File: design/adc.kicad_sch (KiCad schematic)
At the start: 27 parts, among them J6 JUMPER_DFS/GAIN, U12 TLV431ACDBZR, U13 AD9214

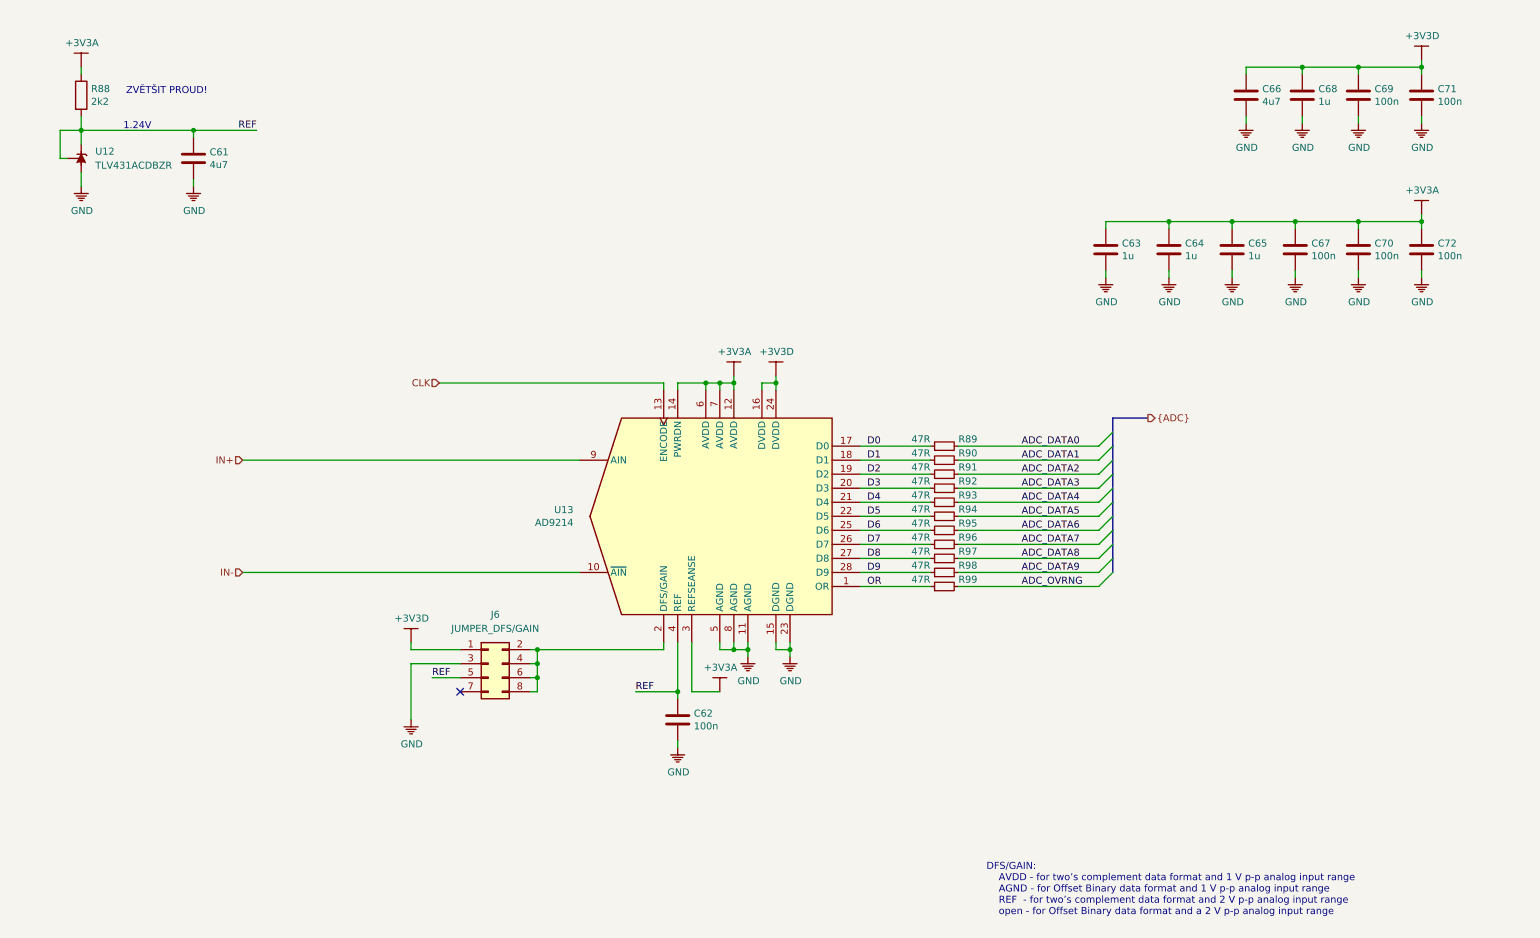
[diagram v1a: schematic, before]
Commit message: Updated schematic
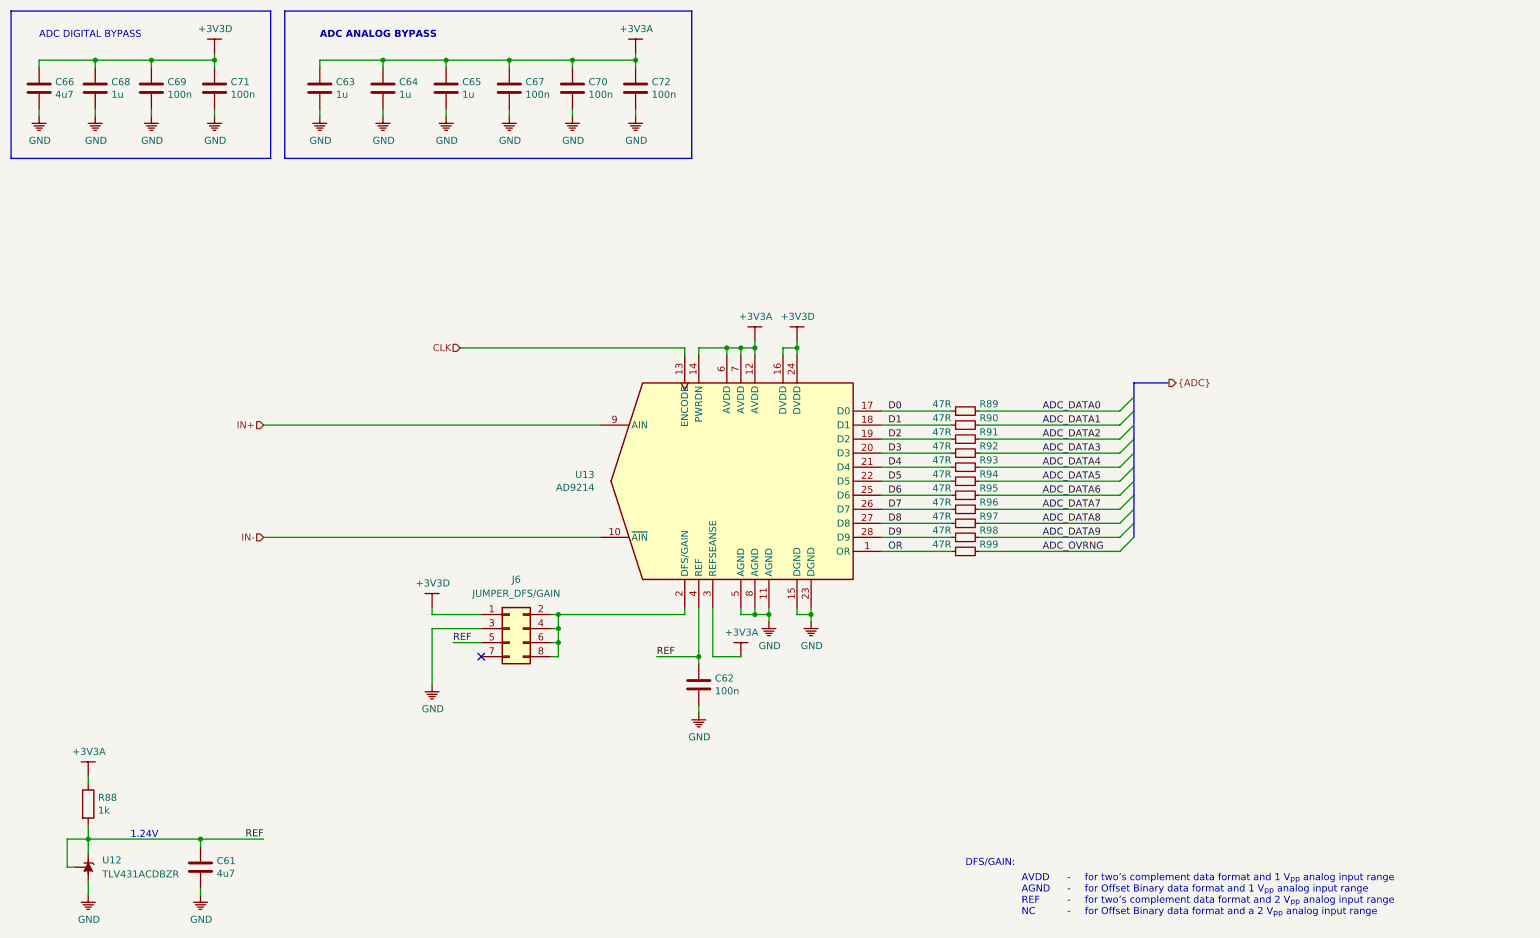
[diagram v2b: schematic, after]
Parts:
- R88: value 2k2 -> 1k
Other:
- note added: "- - - -"
- note added: "ADC ANALOG BYPASS"
- note added: "ADC DIGITAL BYPASS"
- note added: "AVDD AGND REF NC"
- note added: "DFS/GAIN:"
- note added: "for two’s complement data format and 1 V_{pp} analog input range for Offset Binary data format and 1 V_{pp} analog input range for two’s complement data format and 2 V_{pp} analog input range for Offset Binary data format and a 2 V_{pp} analog input range"
- note removed: "DFS/GAIN: AVDD - for two’s complement data format and 1 V p-p analog input range AGND - for Offset Binary data format and 1 V p-p analog input range REF - for two’s complement data format and 2 V p-p analog input range open - for Offset Binary data format and a 2 V p-p analog input range"
- note removed: "ZVĚTŠIT PROUD!"
- moved on the sheet: C61, C62, C63, C64, C65, C66, C67, C68, C69, C70, C71, C72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

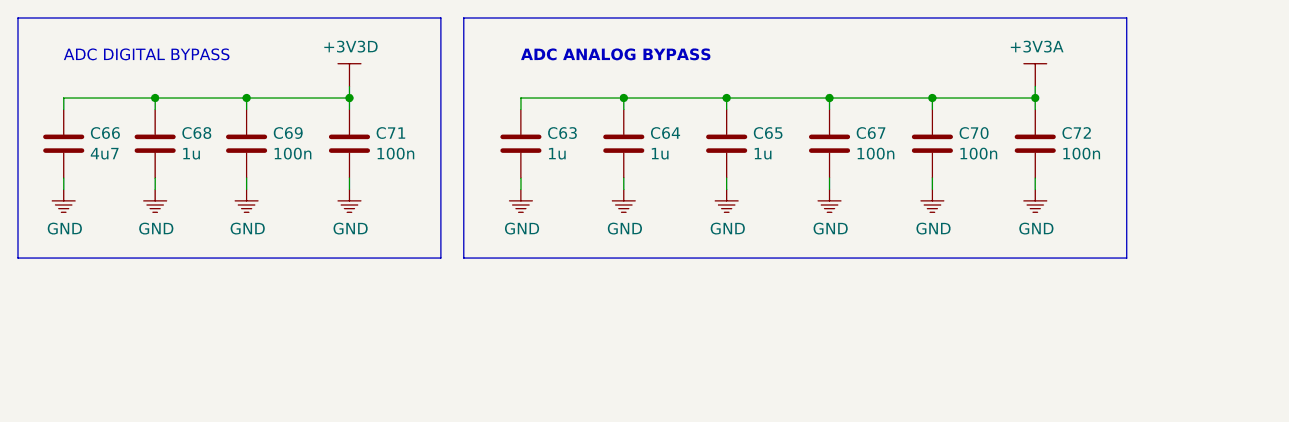
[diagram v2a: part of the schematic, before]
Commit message: Updated LNA
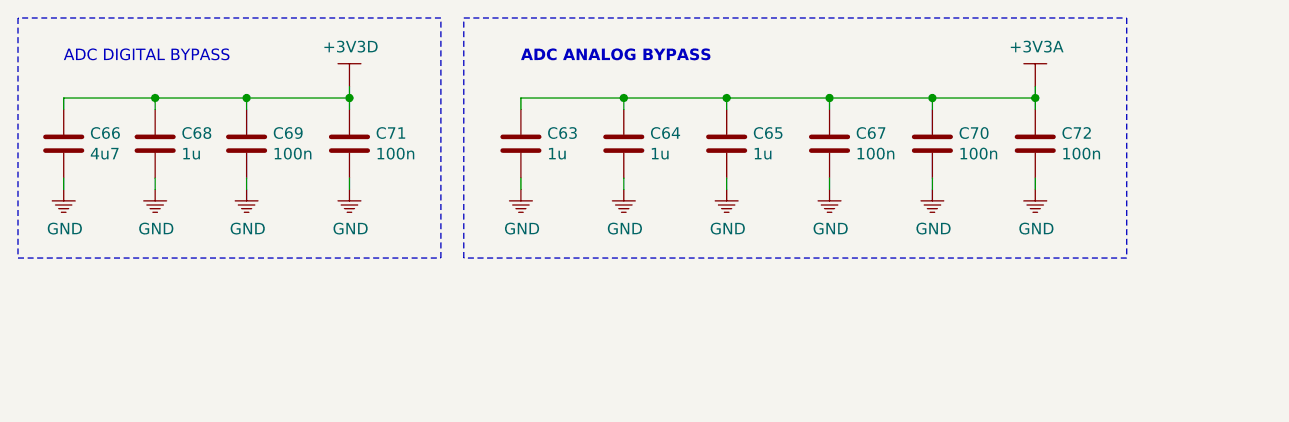
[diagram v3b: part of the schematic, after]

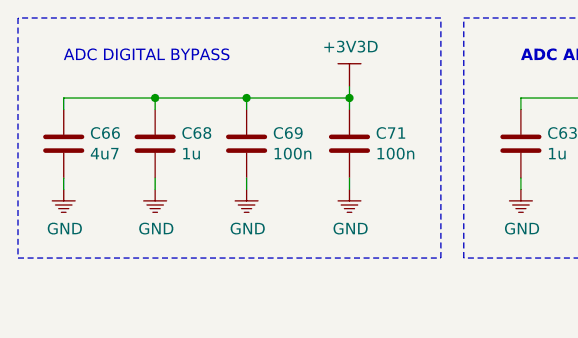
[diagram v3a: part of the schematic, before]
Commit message: Updated notes
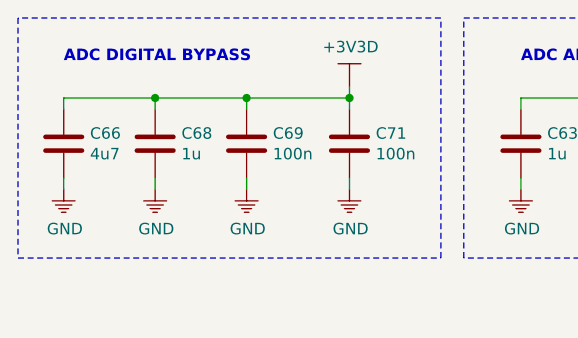
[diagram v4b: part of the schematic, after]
